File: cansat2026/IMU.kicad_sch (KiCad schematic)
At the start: 1 part, among them U701 BNO055 FusionModule

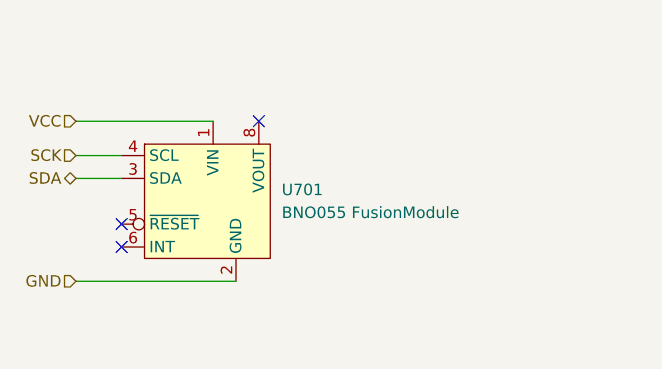
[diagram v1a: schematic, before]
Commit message: Update: いろいろした
無線変えた
カメラのコネクタ変えた
i2cセンサ変えた
電源変えた:1.2V,3.8V,3.3V
IOエキスパンダ追加
FPGA追加
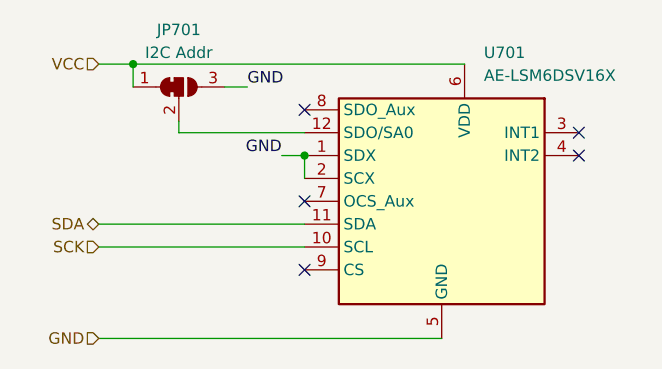
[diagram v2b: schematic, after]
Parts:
- removed U701: BNO055 FusionModule, Project:BNO055-FusionModule, symbol Project:BNO055-FusionModule
- added JP701: I2C Addr, Jumper:SolderJumper-3_P1.3mm_Bridged12_RoundedPad1.0x1.5mm_NumberLabels, symbol Jumper:SolderJumper_3_Bridged12
- added U701: AE-LSM6DSV16X, Project:AE-LSM6DSV16X, symbol Project:AE-LSM6DSV16X
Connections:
- net GND: now also JP701.3 (B), U701.1 (SDX), U701.2 (SCX), U701.5 (GND)
- net SCK: now also U701.10 (SCL)
- net SDA: now also U701.11 (SDA)
- net VCC: now also JP701.1 (A), U701.6 (VDD)
- new net: JP701.2 (C), U701.12 (SDO/SA0)
- no-connect marks 3 -> 5
